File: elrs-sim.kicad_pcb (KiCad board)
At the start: 4 copper layers, 63.5 x 14 mm, 68 parts, among them IC1 SX1280IMLTRT, IC2 ESP8285, J1 Conn_01x04, J10 ESP_TX, J11 GND, J12 3.3V, J13 DP, J14 DN, J2 Conn_01x04, J3 Conn_01x04, J4 VBUS, J6 3.3V_SW, J7 RP_RX, J8 RP_TX, J9 ESP_RX, SW1 SW_SPST, SW2 SW_SPST, U1 RP2040, U2 W25Q16JVSS, X1 SX1M_12MHz, X2 SX1M_26MHz, X3 SX1M_52MHz

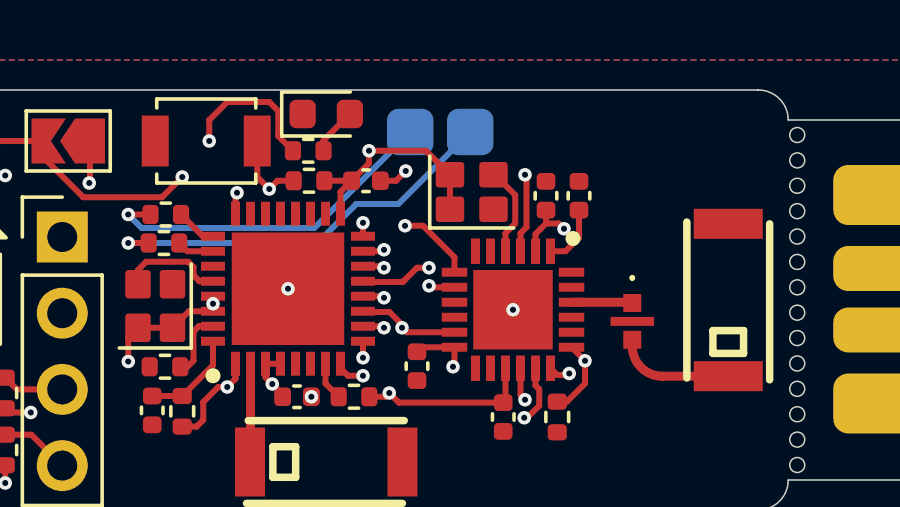
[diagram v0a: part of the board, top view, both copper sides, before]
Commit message: Update: BOM and prod files
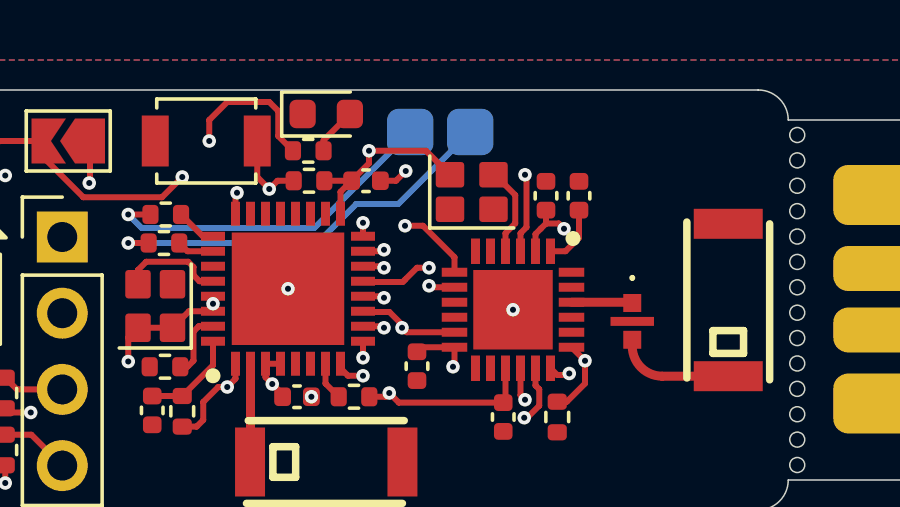
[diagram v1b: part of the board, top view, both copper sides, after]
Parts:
- X3: value SX1M_52MHz -> YSO510TP_52MHz
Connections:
- X3 pad 1: +3.3V_SW -> GND
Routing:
- net +3.3V_SW: track 55.6 -> 54.4 mm
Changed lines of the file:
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@@
 			)
 		)
-		(property "Value" "SX1M_52MHz"
+		(property "Value" "YSO510TP_52MHz"
 			(at 0 2 0)
 			(layer "F.Fab")
@@
 			)
 		)
-		(property "Description" "3.3V HCMOS SMD Crystal Clock Oscillator, Abracon"
+		(property "Description" ""
 			(at 0 0 0)
 			(unlocked yes)
@@
 			(layers "F.Cu" "F.Paste" "F.Mask")
 			(roundrect_rratio 0.12)
-			(net 20 "+3.3V_SW")
-			(pinfunction "EN")
-			(pintype "input")
+			(net 2 "GND")
+			(pinfunction "GND")
+			(pintype "power_in")
 		)
 		(pad "2" smd roundrect
@@
 		(width 0.2)
 		(layer "F.Cu")
-		(net 20)
-	)
-	(segment
-		(start 152.225 105.975)
-		(end 152.225 104.825)
-		(width 0.2)
-		(layer "F.Cu")
